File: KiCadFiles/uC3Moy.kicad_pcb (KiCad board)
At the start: 2 copper layers, 36.1 x 69 mm, 21 parts, among them J1 JACK_INT, J2 JACK, U1 OPA2132, U2 TLE2426

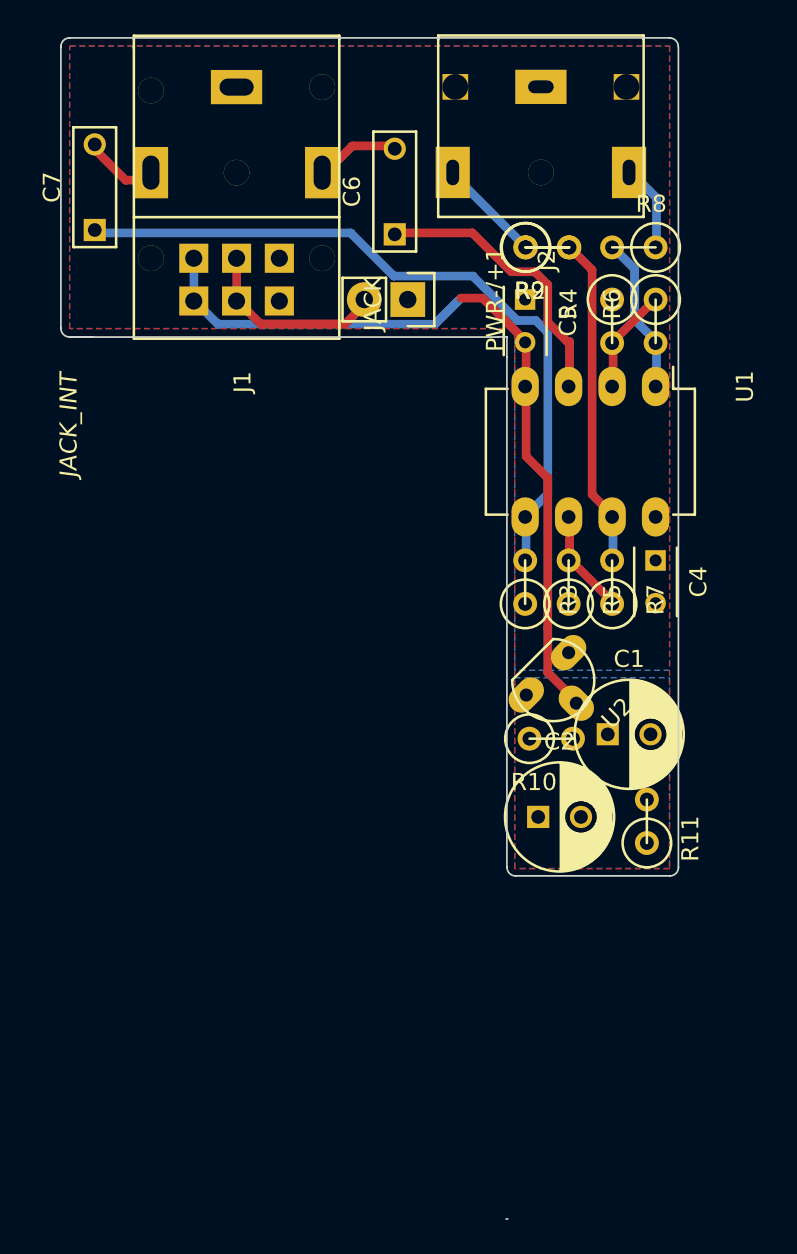
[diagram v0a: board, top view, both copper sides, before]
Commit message: Savepoint
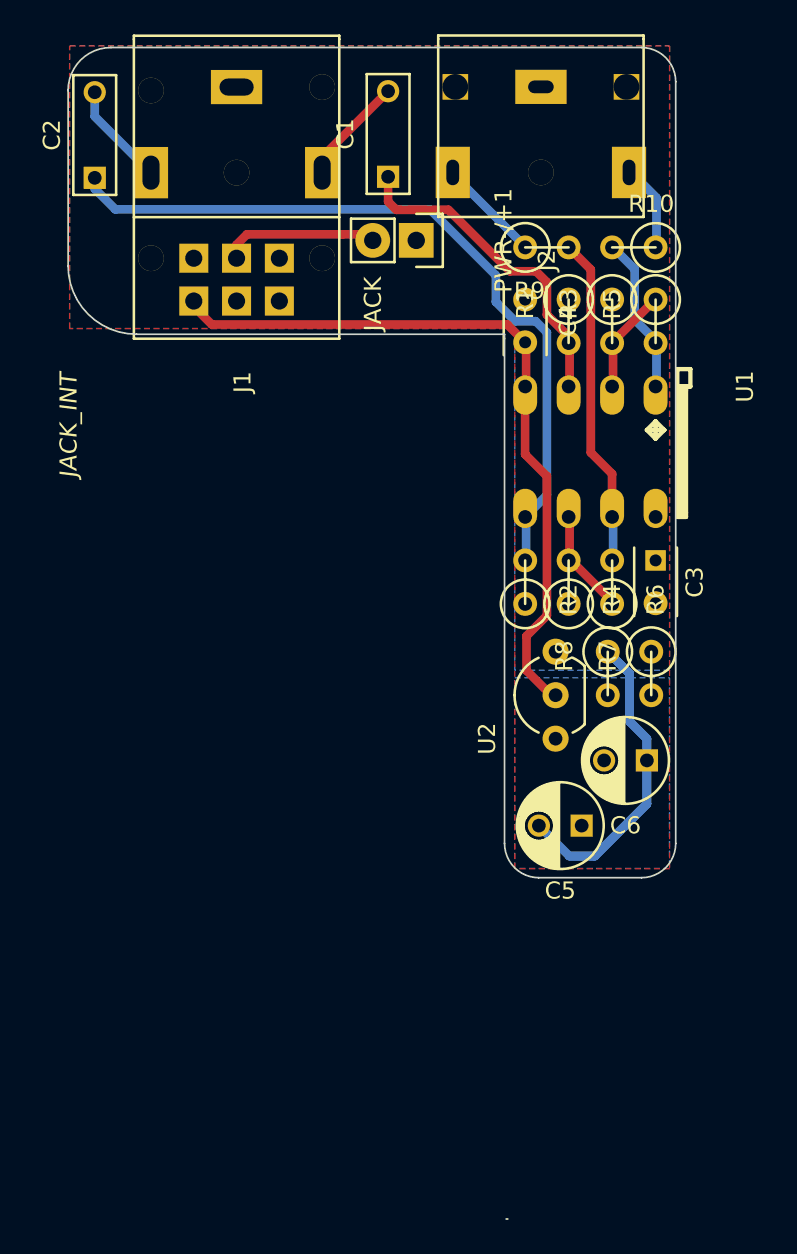
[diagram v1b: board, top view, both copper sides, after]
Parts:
- removed C7: 1 uF, Capacitors_ThroughHole:C_Rect_L7_W2.5_P5
- removed R11: R, Discret:R1
- added C3: C, Capacitors_ThroughHole:C_Rect_L4_W2.5_P2.5, F.Cu at (242.8, 156.5)
- added G***: LOGO, uc3music_logos:logo_pick_6x6mm, B.Cu at (239.2, 150.5)
- added G***: LOGO, uc3music_logos:logo_guitar_22.5x7.7mm, B.Cu at (239.8, 163.5)
- added R1: R, Discret:R1, F.Cu at (237.7, 142.5)
- C1, C2: value CAPAPOL -> 1 uF; footprint Capacitors_ThroughHole:C_Radial_D6.3_L11.2_P2.5 -> Capacitors_ThroughHole:C_Rect_L7_W2.5_P5
- C5: value C -> CP; footprint Capacitors_ThroughHole:C_Rect_L4_W2.5_P2.5 -> Capacitors_ThroughHole:C_Radial_D5_L6_P2.5
- C6: value 1 uF -> CP; footprint Capacitors_ThroughHole:C_Rect_L7_W2.5_P5 -> Capacitors_ThroughHole:C_Radial_D5_L6_P2.5
- U1: footprint Housings_DIP:DIP-8_W7.62mm_LongPads -> uC3Moy:DIP-8_W7.62mm_jorfru
- U2: footprint uC3Moy:TO-92_JorFru_compact -> Housings_TO-92:TO-92_Inline_Wide
- moved C2 45.4 mm to (210.1, 134.1), turned to 90 degrees
- moved C1 35.0 mm to (227.2, 134.1), turned to 90 degrees
- moved C6 34.1 mm to (242.3, 168.1), turned to 180 degrees
- moved C5 30.9 mm to (238.5, 172.0), turned to 180 degrees
- moved R10 29.1 mm to (241.6, 138.2), turned to 180 degrees
- moved R8 24.9 mm to (240.0, 163.1), turned to 270 degrees
- moved R2 19.6 mm to (235.2, 157.7), turned to 90 degrees
- moved C4 17.0 mm to (235.2, 141.2)
- moved R5 16.1 mm to (242.8, 142.5), turned to 270 degrees
- moved R3 16.1 mm to (240.3, 142.5), turned to 270 degrees
- moved R6 15.5 mm to (240.3, 157.7), turned to 90 degrees
- moved R4 15.5 mm to (237.7, 157.7), turned to 90 degrees
- moved R7 5.80 mm to (242.6, 163.1), turned to 270 degrees
- moved U2 4.38 mm to (237.0, 166.9), turned to 90 degrees
- moved PWR-/+1 3.49 mm to (228.8, 137.8)
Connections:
- C1 pad 1: +6V -> Net-(C1-Pad1)
- C1 pad 2: GND -> Net-(C1-Pad2)
- C2 pad 1: GND -> Net-(C2-Pad1)
- C2 pad 2: -6V -> Net-(C2-Pad2)
- C4 pad 1: +6V -> GND
- C4 pad 2: GND -> -6V
- C5 pad 1: GND -> +6V
- C5 pad 2: -6V -> GND
- C6 pad 1: Net-(C6-Pad1) -> GND
- C6 pad 2: Net-(C6-Pad2) -> -6V
- J1 pad 3: Net-(C7-Pad2) -> Net-(C2-Pad2)
- J1 pad 4: Net-(C6-Pad2) -> Net-(C1-Pad2)
- R10 pad 1: +6V -> Net-(J2-Pad4)
- R10 pad 2: GND -> Net-(R10-Pad2)
- R2 pad 2: Net-(C6-Pad1) -> Net-(C2-Pad1)
- R3 pad 2: Net-(C7-Pad1) -> Net-(R3-Pad2)
- R5 pad 1: GND -> Net-(R3-Pad2)
- R5 pad 2: Net-(R5-Pad2) -> Net-(R10-Pad2)
- R7 pad 1: Net-(R5-Pad2) -> GND
- R7 pad 2: Net-(R7-Pad2) -> +6V
- R8 pad 1: Net-(J2-Pad4) -> GND
- R8 pad 2: Net-(R6-Pad2) -> -6V
- R9 pad 2: Net-(R7-Pad2) -> Net-(R6-Pad2)
- U1 pad 1: Net-(R6-Pad2) -> Net-(R10-Pad2)
- U1 pad 2: Net-(R4-Pad2) -> Net-(R3-Pad2)
- U1 pad 3: Net-(C6-Pad1) -> Net-(C1-Pad1)
- U1 pad 5: Net-(C7-Pad1) -> Net-(C2-Pad1)
- U1 pad 6: Net-(R5-Pad2) -> Net-(R4-Pad2)
- U1 pad 7: Net-(R7-Pad2) -> Net-(R6-Pad2)
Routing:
- net Net-(C2-Pad1): track 0.00 -> 45.3 mm
- net Net-(C7-Pad1): track 42.8 -> 0.00 mm
- net GND: track 0.00 -> 33.8 mm
- net Net-(C1-Pad1): track 0.00 -> 19.4 mm
- net Net-(R7-Pad2): track 19.3 -> 0.00 mm
- net Net-(C6-Pad1): track 16.6 -> 0.00 mm
- net Net-(R6-Pad2): track 9.10 -> 19.3 mm
- net Net-(R10-Pad2): track 0.00 -> 9.10 mm
- net Net-(C1-Pad2): track 0.00 -> 6.76 mm
- net Net-(R3-Pad2): track 0.00 -> 6.13 mm
- net Net-(R5-Pad2): track 6.13 -> 0.00 mm
- net Net-(C2-Pad2): track 0.00 -> 6.06 mm
- net Net-(C6-Pad2): track 5.20 -> 0.00 mm
- net Net-(C7-Pad2): track 4.17 -> 0.00 mm
- net -6V: track 45.9 -> 43.1 mm
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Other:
- board size 36.1 x 69 mm -> 35.5 x 68.4 mm
- board text added: "by: JorFru"
- board text added: "v1.1"
- board text removed: "v1.0"

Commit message: Ready to rock
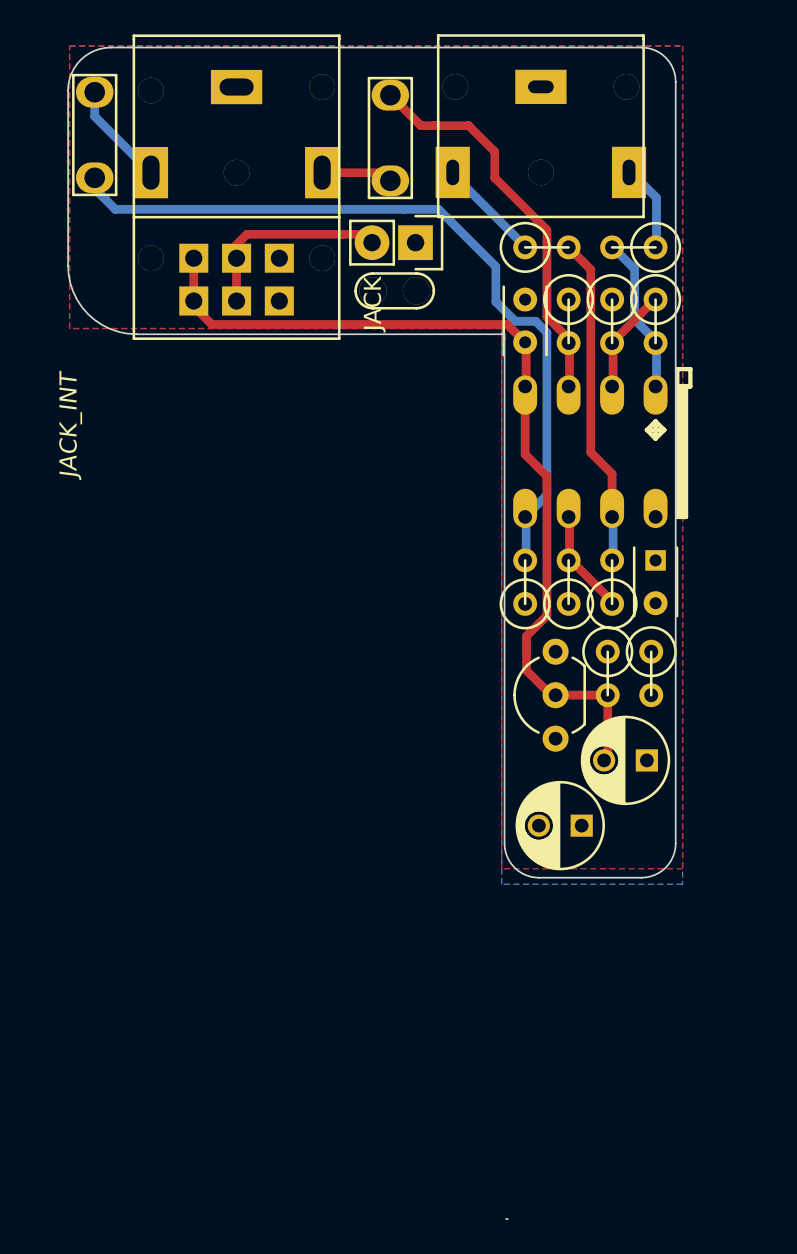
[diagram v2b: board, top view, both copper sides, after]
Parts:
- added REF**: Test_Point, Measurement_Points:Test_Point, F.Cu at (227.6, 140.7)
- added REF**: Symbol_OSHW-Logo_SilkScreen, uC3Moy:Symbol_OSHW-Logo_SilkScreen_compact, B.Cu at (241.0, 128.8)
- moved C1 4.77 mm to (227.3, 129.3), turned to 270 degrees
- moved PWR-/+1 0.14 mm to (228.8, 137.9)
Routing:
- net GND: track 33.8 -> 0.00 mm
- net -6V: track 43.1 -> 52.8 mm
- net Net-(C1-Pad1): track 19.4 -> 23.5 mm
- net Net-(J1-Pad1): track 9.15 -> 11.6 mm
- net Net-(C1-Pad2): track 6.76 -> 5.49 mm
- removed copper zone on B.Cu, net -6V
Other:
- board text added: "UC3Music"
- board text removed: "UC3Music-e"
